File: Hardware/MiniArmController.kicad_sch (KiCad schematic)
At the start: 7 parts, among them U1 Teensy4.1_DEV-16771

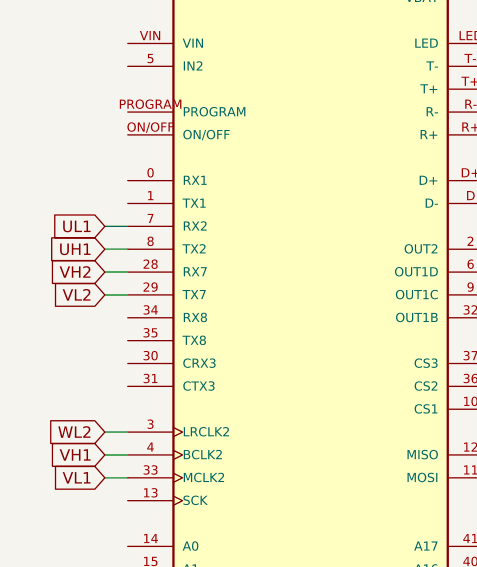
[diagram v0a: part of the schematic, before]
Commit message: Superseded changes
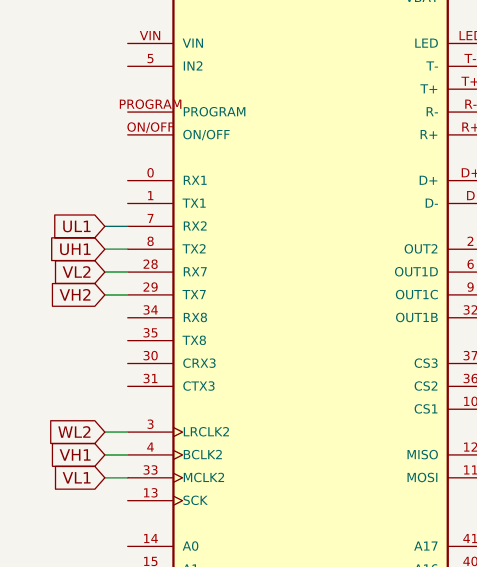
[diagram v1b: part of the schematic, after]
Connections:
- net VH2: now also U1.29 (TX7); no longer U1.28 (RX7)
- net VL2: now also U1.28 (RX7); no longer U1.29 (TX7)
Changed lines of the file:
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@@
+	(wire
+		(pts
+			(xy 53.34 74.93) (xy 55.88 74.93)
+		)
+		(stroke
+			(width 0)
+			(type default)
+		)
+	)
 	(wire
 		(pts
@@
 	(wire
 		(pts
-			(xy 53.34 74.93) (xy 55.88 74.93)
-		)
-		(stroke
-			(width 0)
-			(type default)
-		)
-	)
-	(wire
-		(pts
 			(xy 190.5 92.71) (xy 193.04 92.71)
 		)
@@
 	(wire
 		(pts
+			(xy 53.34 77.47) (xy 55.88 77.47)
+		)
+		(stroke
+			(width 0)
+			(type default)
+		)
+	)
+	(wire
+		(pts
 			(xy 190.5 55.88) (xy 193.04 55.88)
 		)
@@
 		(pts
 			(xy 210.82 60.96) (xy 208.28 60.96)
-		)
-		(stroke
-			(width 0)
-			(type default)
-		)
-	)
-	(wire
-		(pts
-			(xy 53.34 77.47) (xy 55.88 77.47)
 		)
 		(stroke
@@
 	(global_label "VH2"
 		(shape input)
-		(at 53.34 74.93 180)
+		(at 53.34 77.47 180)
 		(fields_autoplaced yes)
 		(effects
@@
 		)
 		(property "Intersheetrefs" "${INTERSHEET_REFS}"
-			(at 46.7262 74.93 0)
+			(at 46.7262 77.47 0)
 			(effects
 				(font
@@
 	(global_label "VL2"
 		(shape input)
-		(at 53.34 77.47 180)
+		(at 53.34 74.93 180)
 		(fields_autoplaced yes)
 		(effects
@@
 		)
 		(property "Intersheetrefs" "${INTERSHEET_REFS}"
-			(at 47.0286 77.47 0)
+			(at 47.0286 74.93 0)
 			(effects
 				(font
